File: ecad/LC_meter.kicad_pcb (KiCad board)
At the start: 2 copper layers, 77.7 x 77 mm, 75 parts, among them J1 DUT, J10 Range Switch, J11 Range Switch, J12 Display Connector, J2 Switch, J3 12V Power, J4 Switch, J6 Switch, J7 Switch, J8 Thevenin Range Switch Indicat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, J9 Current Range Switch Indicator, U1 LM6144xIx, U2 LM4030-4.096, U3 Raspberry Pi Pico SC0915, U4 ADS8328IPW, U5 LM1117DT-3.3, U8 LM1117DT-5.0

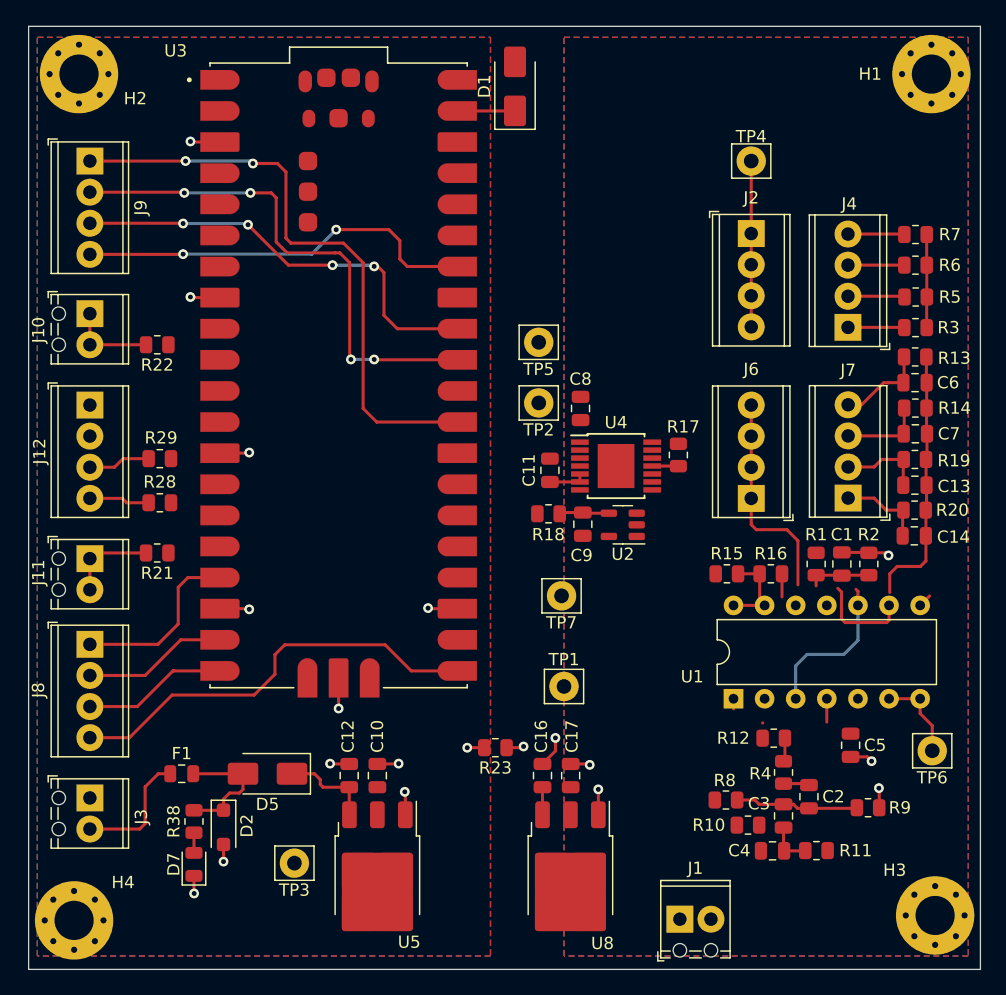
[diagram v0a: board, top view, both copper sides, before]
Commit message: layout
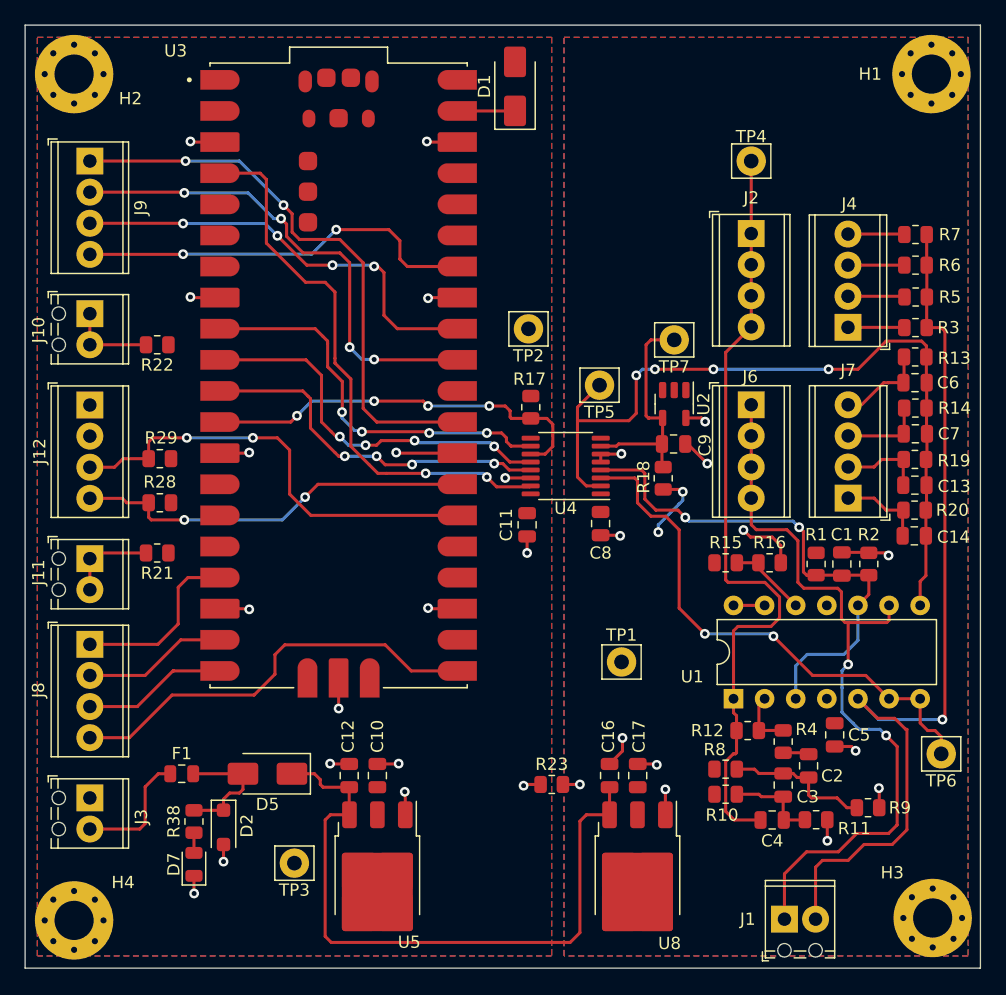
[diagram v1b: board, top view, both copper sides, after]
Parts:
- U4: footprint Package_SO:TSSOP-14-1EP_4.4x5mm_P0.65mm -> Package_SO:TSSOP-16_4.4x5mm_P0.65mm
- moved TP7 22.8 mm to (154.0, 81.7)
- moved R17 12.7 mm to (142.3, 87.2)
- moved U2 10.7 mm to (154.0, 86.9), turned to -90 degrees
- moved C9 9.89 mm to (153.9, 90.2), turned to 0 degrees
- moved R18 9.80 mm to (153.1, 93.0), turned to 90 degrees
- moved C8 9.54 mm to (148.0, 96.7), turned to -90 degrees
- moved J1 8.54 mm to (163.0, 129.0)
- moved J6 7.64 mm to (160.3, 87.0), turned to -90 degrees
- moved TP2 6.11 mm to (142.1, 80.8)
- moved TP5 6.07 mm to (147.9, 85.4)
- moved R23 5.49 mm to (144.0, 118.0), turned to 0 degrees
- moved C17 5.48 mm to (151.0, 117.3)
- moved C16 5.47 mm to (148.7, 117.3)
- moved U8 5.47 mm to (151.0, 125.5)
- moved TP1 5.11 mm to (149.7, 108.0)
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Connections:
- C11 pad 2: GNDA -> GNDD
- J12 pad 1: +5V -> +3.3V
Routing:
- net Net-(J1-Pin_2): track 7.61 -> 74.8 mm, vias 0 -> 1
- net Net-(J2-Pin_1): track 14.4 -> 64.4 mm
- net /Analog Front End/SCK: track 0.00 -> 45.7 mm, vias 0 -> 2
- net Net-(D5-K): track 9.87 -> 54.6 mm
- net Net-(U4-+IN1): track 22.8 -> 65.1 mm, vias 0 -> 4
- net Net-(J1-Pin_1): track 25.6 -> 63.0 mm, vias 0 -> 2
- net Net-(U1B--): track 7.20 -> 43.9 mm, vias 0 -> 2
- net /Analog Front End/INTERUPT: track 0.00 -> 32.5 mm, vias 0 -> 4
- net /SDA: track 5.09 -> 36.5 mm, vias 0 -> 2
- net /Analog Front End/DATA_IN: track 0.00 -> 31.4 mm, vias 0 -> 4
- net /Analog Front End/CS: track 2.14 -> 32.8 mm, vias 0 -> 4
- net /Analog Front End/DATA_OUT: track 0.00 -> 29.7 mm, vias 0 -> 4
- net /SCL: track 4.95 -> 32.6 mm, vias 0 -> 2
- net /Analog Front End/V/2: track 18.1 -> 43.0 mm, vias 0 -> 2
- net Net-(U2-K): track 4.07 -> 18.9 mm
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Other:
- board size 77.7 x 77 mm -> 78 x 77 mm
